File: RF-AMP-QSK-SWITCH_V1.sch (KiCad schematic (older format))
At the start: 41 parts, among them J1 TRX, J2 AMP_IN, J3 ANT, J4 AMP_OUT

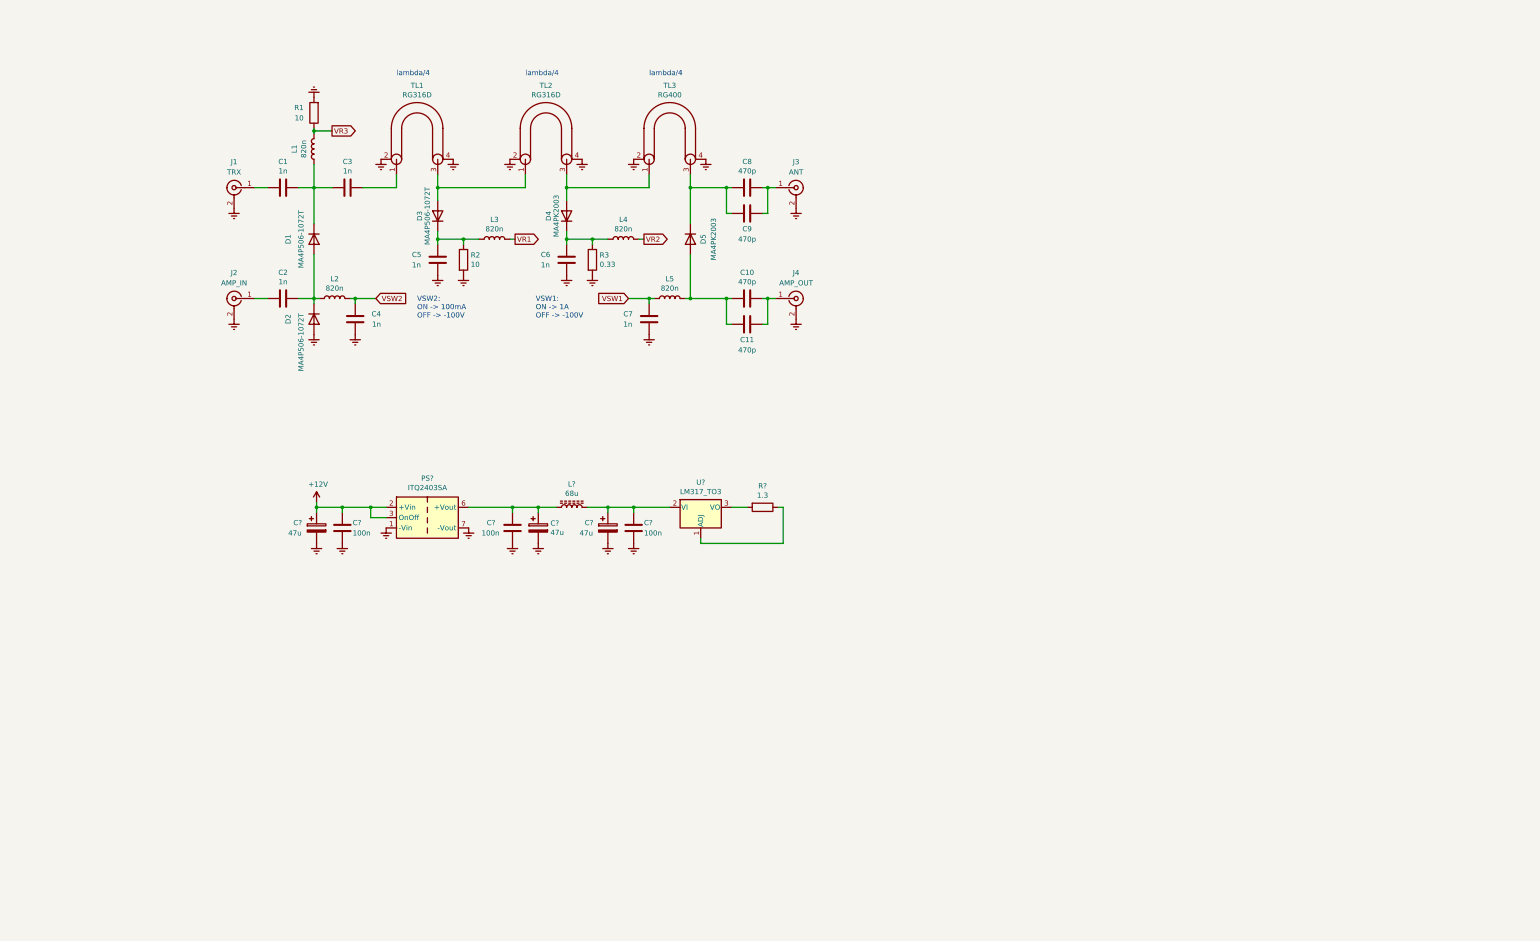
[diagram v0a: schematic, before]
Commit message: initial commit
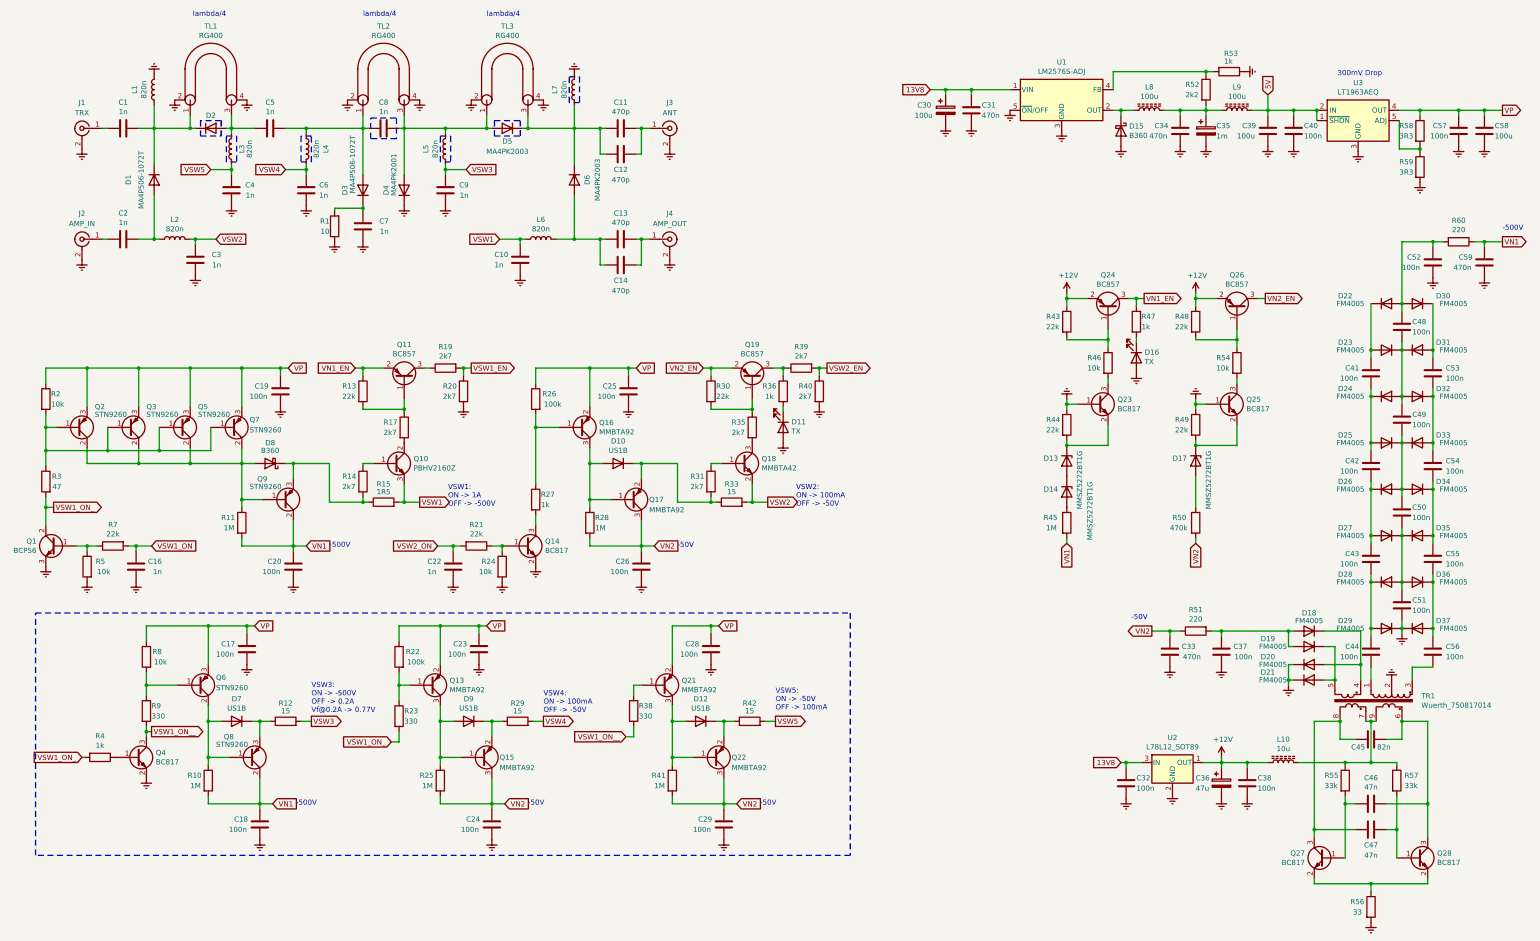
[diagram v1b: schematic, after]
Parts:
- removed C?: 47u, symbol Device:CP
- removed C?: 100n, symbol Device:C
- removed L?: 68u, symbol Device:L_Core_Ferrite
- removed PS?: ITQ2403SA, Converter_DCDC:Converter_DCDC_XP_POWER-ITxxxxxS_THT, symbol Converter_DCDC:ITQ2403SA
- removed R?: 1.3, symbol Device:R
- removed U?: LM317_TO3, Package_TO_SOT_THT:TO-3, symbol Regulator_Linear:LM317_TO3
- added C16, C22: 1n, Capacitor_SMD:C_0805_2012Metric, symbol Device:C
- added C17, C19, C23, C24, C25, C26, C28, C29, C32, C38, C40, C57: 100n, Capacitor_SMD:C_0805_2012Metric, symbol Device:C
- added C18, C20, C37, C41, C42, C43, C44, C48, C49, C50, C51, C52, C53, C54, C55, C56: 100n, Capacitor_SMD:C_1206_3216Metric, symbol Device:C
- added C33, C59: 470n, Capacitor_SMD:C_1206_3216Metric, symbol Device:C
- added C36: 47u, Capacitor_SMD:CP_Elec_10x10, symbol Device:CP
- added C39, C58: 100u, Capacitor_SMD:C_1210_3225Metric, symbol Device:C
- added C4, C7, C9: 1n, Capacitor_SMD:C_1210_3225Metric, symbol Device:C
- added C45: 82n, Capacitor_SMD:C_0805_2012Metric, symbol Device:C
- added C46, C47: 47n, Capacitor_SMD:C_0805_2012Metric, symbol Device:C
- added D10, D12, D7, D9: US1B, Diode_SMD:D_SMA, symbol Diode:US1B
- added D11, D16: TX, LED_THT:LED_D3.0mm, symbol Device:LED
- added D13, D14, D17: MMSZ5272BT1G, Diode_SMD:D_SOD-123, symbol Diode:BZD27Cxx
- added D15, D8: B360, Diode_SMD:D_SMC, symbol Diode:B360
- added D18, D19, D20, D21, D22, D23, D24, D25, D26, D27, D28, D29, D30, D31, D32, D33, D34, D35, D36, D37: FM4005, Diode_SMD:D_SMA, symbol Diode:MRA4006T3G
- added D5: MA4PK2003, RF-AMP-QSK-SWITCH_V1:MA4PK200x, symbol Device:D
- added L10: 10u, Inductor_SMD:L_1210_3225Metric, symbol Device:L_Core_Ferrite
- added L5, L7: 820n, RF-AMP-QSK-SWITCH_V1:Air_Coil_1, symbol Device:L
- added L8, L9: 100u, Inductor_SMD:L_Bourns_SRR1210A, symbol Device:L_Core_Ferrite
- added Q1: BCP56, Package_TO_SOT_SMD:SOT-223-3_TabPin2, symbol Transistor_BJT:BCP56
- added Q10: PBHV2160Z, Package_TO_SOT_SMD:SOT-223-3_TabPin2, symbol Transistor_BJT:PZTA42
- added Q11, Q19, Q24, Q26: BC857, Package_TO_SOT_SMD:SOT-23, symbol Transistor_BJT:BC857
- added Q13, Q15, Q16, Q17, Q21, Q22: MMBTA92, Package_TO_SOT_SMD:SOT-23, symbol Transistor_BJT:MMBTA92
- added Q14, Q23, Q25, Q27, Q28, Q4: BC817, Package_TO_SOT_SMD:SOT-23, symbol Transistor_BJT:BC817
- added Q18: MMBTA42, Package_TO_SOT_SMD:SOT-23, symbol Transistor_BJT:MMBTA42
- added Q2, Q3, Q5, Q6, Q7, Q8, Q9: STN9260, Package_TO_SOT_SMD:SOT-223-3_TabPin2, symbol Transistor_BJT:BD912
- added R10, R11, R25, R28, R41, R45: 1M, Resistor_SMD:R_0805_2012Metric, symbol Device:R
- added R12, R29, R33, R42: 15, Resistor_SMD:R_2512_6332Metric, symbol Device:R
- added R13, R21, R30, R43, R44, R48, R49, R7: 22k, Resistor_SMD:R_0805_2012Metric, symbol Device:R
- added R14, R17, R19, R20, R31, R35, R39, R40: 2k7, Resistor_SMD:R_0805_2012Metric, symbol Device:R
- added R15: 1R5, Resistor_SMD:R_Shunt_Vishay_WSR2_WSR3, symbol Device:R
- added R22, R26: 100k, Resistor_SMD:R_0805_2012Metric, symbol Device:R
- added R23, R38, R9: 330, Resistor_SMD:R_0805_2012Metric, symbol Device:R
- added R24, R46, R5, R54, R8: 10k, Resistor_SMD:R_0805_2012Metric, symbol Device:R
- added R27, R36, R4, R47, R53: 1k, Resistor_SMD:R_0805_2012Metric, symbol Device:R
- added R50: 470k, Resistor_SMD:R_0805_2012Metric, symbol Device:R
- added R51, R60: 220, Resistor_SMD:R_0805_2012Metric, symbol Device:R
- added R52: 2k2, Resistor_SMD:R_0805_2012Metric, symbol Device:R
- added R55, R57: 33k, Resistor_SMD:R_0805_2012Metric, symbol Device:R
- added R56: 33, Resistor_SMD:R_0805_2012Metric, symbol Device:R
- added R58, R59: 3R3, Resistor_SMD:R_0805_2012Metric, symbol Device:R
- added TR1: Wuerth_750817014, RF-AMP-QSK-SWITCH_V1:Transformer_Wuerth_750817014, symbol RF-AMP:Wuerth_750817014
- added U1: LM2576S-ADJ, Package_TO_SOT_SMD:TO-263-5_TabPin3, symbol Regulator_Switching:LM2576S-ADJ
- added U2: L78L12_SOT89, Package_TO_SOT_SMD:SOT-89-3, symbol Regulator_Linear:L78L12_SOT89
- added U3: LT1963AEQ, Package_TO_SOT_SMD:TO-263-5_TabPin3, symbol Regulator_Linear:LT1963AEQ
- C1, C2, C5, C6: footprint (none) -> Capacitor_SMD:C_1210_3225Metric
- C10: renamed from C7; footprint (none) -> Capacitor_SMD:C_1210_3225Metric
- C11: renamed from C8; footprint (none) -> Capacitor_SMD:C_1210_3225Metric
- C12: renamed from C9; footprint (none) -> Capacitor_SMD:C_1210_3225Metric
- C13: renamed from C10; footprint (none) -> Capacitor_SMD:C_1210_3225Metric
- C14: renamed from C11; footprint (none) -> Capacitor_SMD:C_1210_3225Metric
- C3: renamed from C4; footprint (none) -> Capacitor_SMD:C_1210_3225Metric
- C30: renamed from C?; value 47u -> 100u; footprint (none) -> Capacitor_SMD:CP_Elec_10x10
- C31, C34: renamed from C?; value 100n -> 470n; footprint (none) -> Capacitor_SMD:C_0805_2012Metric
- C35: renamed from C?; value 47u -> 1m; footprint (none) -> Capacitor_SMD:CP_Elec_10x10
- C8: renamed from C3; footprint (none) -> Capacitor_SMD:C_1210_3225Metric
- D1, D2, D3: footprint (none) -> Diode_SMD:D_1210_3225Metric
- D4: value MA4PK2003 -> MA4PK2001; footprint (none) -> RF-AMP-QSK-SWITCH_V1:MA4PK200x
- D6: renamed from D5; footprint (none) -> RF-AMP-QSK-SWITCH_V1:MA4PK200x
- J1, J2, J3, J4: footprint (none) -> RF-AMP-QSK-SWITCH_V1:N_connector_panel_small_flange
- L1, L2, L3, L4: footprint (none) -> RF-AMP-QSK-SWITCH_V1:Air_Coil_1
- L6: renamed from L5; footprint (none) -> RF-AMP-QSK-SWITCH_V1:Air_Coil_1
- R1: footprint (none) -> Resistor_SMD:R_1210_3225Metric
- R2: value 10 -> 10k; footprint (none) -> Resistor_SMD:R_0805_2012Metric
- R3: value 0.33 -> 47; footprint (none) -> Resistor_SMD:R_1206_3216Metric
- TL1, TL2: value RG316D -> RG400
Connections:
- net VR2 is gone; now on an unnamed net: L4.2
- net VR3 is gone; now on net Earth: L1.2, R1.1
- net +12V: now also C36.1, C38.2, L10.1, Q24.2 (E), Q26.2 (E), R43.1, R48.1, U2.1 (OUT); no longer C30.1, C31.2
- net Earth: now also D4.1 (K), C16.1, C17.1, C18.1, C19.1, C20.1, C22.1, C23.1, C24.1, C25.1, C26.1, C28.1, C29.1, C32.1, C33.1, C36.2, C37.1, C38.1, C39.1, C4.1, C40.1, C51.1, C52.1, C57.1, C58.1, C59.1, C7.1, C9.1, D11.2 (A), D15.2 (A), D16.2 (A), D20.1 (K), D21.1 (K), D29.1 (K), D37.1 (K), L7.2, Q1.3 (E), Q14.2 (E), Q23.1 (B), Q25.1 (B), Q4.2 (E), R20.2, R24.2, R40.2, R44.1, R49.1, R5.2, R53.1, R56.2, R59.2, TR1.2, U1.3 (GND), U1.5 (~ON~/OFF), U2.2 (GND), U3.3 (GND); no longer C5.1, D2.2 (A), R1.2, R2.2, R3.2
- net VSW1: now also Q10.3 (E), R15.2
- net VSW2: now also Q18.2 (E), R33.2
- net at C11.1, C12.1, D6.1 (K)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: now also D5.1 (K), L7.1
- net at C1.1, D1.1 (K), L1.1: now also D2.1 (K), TL1.1 (IC1); no longer C8.2
- net at C8.1: now also D4.2 (A), TL2.3 (IC1), TL3.1 (IC1), D5.2 (A), L5.2; no longer TL1.1 (IC1)
- net at D3.2 (A), TL2.1 (IC1): now also C5.1, C8.2; no longer TL1.3 (IC1)
- net VSW4: now reaches C6.2, L4.1
- net VSW4: now also R29.2; no longer D4.1 (K), R3.1
- net at C2.1, D1.2 (A), L2.2: no longer D2.1 (K)
- net at C34.2, C35.1: now also L8.2, L9.1, R52.2
- net VR1: no longer names the net of L3.2
- net VR1: now also C5.2, D2.2 (A), TL1.3 (IC1)
- new net: C7.2, D3.1 (K), R1.2
- new net: D15.1 (K), L8.1, U1.2 (OUT)
- new net: C55.1, C56.2, D36.1 (K), D37.2 (A)
- new net: R58.2, R59.1, U3.5 (ADJ)
- new net: Q27.2 (E), Q28.2 (E), R56.1
- new net: C44.1, TR1.1
- new net: C56.1, TR1.3
- new net: D18.1 (K), D20.2 (A), TR1.4
- new net: D19.1 (K), D21.2 (A), TR1.5
- new net: C45.1, C46.1, Q28.3 (C), TR1.6
- new net: L10.2, R55.1, R57.1, TR1.7, TR1.9
- new net: C45.2, C47.2, Q27.3 (C), TR1.8
- new net: Q2.1 (B), Q3.1 (B), Q5.1 (B), Q7.1 (B), R2.2, R3.1
- new net: D8.2 (A), Q2.2 (C), Q3.2 (C), Q5.2 (C), Q7.2 (C), Q9.1 (B), R11.1
- new net: D8.1 (K), Q9.3 (E), R14.2, R15.1
- new net: Q1.1 (B), R5.1, R7.1
- new net: R52.1, R53.2, U1.4 (FB)
- new net: C47.1, Q28.1 (B), R57.2
- new net: C37.2, D18.2 (A), D19.2 (A), R51.2
- new net: C46.2, Q27.1 (B), R55.2
- new net: C48.2, C52.2, D22.2 (A), D30.2 (A), R60.2
- new net: Q19.3 (C), R36.1, R39.1
- new net: D11.1 (K), R36.2
- new net: D13.1 (K), Q23.2 (E), R44.2
- new net: D13.2 (A), D14.1 (K)
- new net: Q11.1 (B), R13.2, R17.1
- new net: Q24.1 (B), R43.2, R46.1
- new net: Q23.3 (C), R46.2
- new net: D16.1 (K), R47.2
- new net: Q10.1 (B), R14.1
- new net: Q10.2 (C), R17.2
- new net: D14.2 (A), R45.1
- new net: D10.2 (A), Q16.3 (C), Q17.1 (B), R28.1
- new net: Q14.1 (B), R21.1, R24.1
- new net: Q16.1 (B), R26.2, R27.1
- new net: Q14.3 (C), R27.2
- new net: Q11.3 (C), R19.1
- new net: C43.1, C44.2, D28.1 (K), D29.2 (A)
- new net: D10.1 (K), Q17.2 (E), R31.2, R33.1
- new net: Q18.1 (B), R31.1
- new net: Q19.1 (B), R30.2, R35.1
- new net: Q18.3 (C), R35.2
- new net: D17.1 (K), Q25.2 (E), R49.2
- new net: D17.2 (A), R50.1
- new net: Q26.1 (B), R48.2, R54.1
- new net: Q25.3 (C), R54.2
- new net: C50.1, C51.2, D27.1 (K), D28.2 (A), D35.1 (K), D36.2 (A)
- new net: D7.2 (A), Q6.2 (C), Q8.1 (B), R10.1
- new net: Q4.1 (B), R4.1
- new net: D7.1 (K), Q8.3 (E), R12.1
- new net: Q6.1 (B), R8.2, R9.1
- new net: C54.1, C55.2, D34.1 (K), D35.2 (A)
- new net: C42.1, C43.2, D26.1 (K), D27.2 (A)
- new net: C49.1, C50.2, D25.1 (K), D26.2 (A), D33.1 (K), D34.2 (A)
- new net: C53.1, C54.2, D32.1 (K), D33.2 (A)
- new net: C41.1, C42.2, D24.1 (K), D25.2 (A)
- new net: C48.1, C49.2, D23.1 (K), D24.2 (A), D31.1 (K), D32.2 (A)
- new net: C53.2, D30.1 (K), D31.2 (A)
- new net: C41.2, D22.1 (K), D23.2 (A)
- new net: D9.2 (A), Q13.3 (C), Q15.1 (B), R25.1
- new net: Q13.1 (B), R22.2, R23.1
- new net: D9.1 (K), Q15.2 (E), R29.1
- new net: D12.2 (A), Q21.3 (C), Q22.1 (B), R41.1
- new net: Q21.1 (B), R38.1
- new net: D12.1 (K), Q22.2 (E), R42.1
- new net 13V8: C30.1, C31.2, C32.2, U1.1 (VIN), U2.3 (IN)
- new net 5V: C39.2, C40.2, L9.2, U3.1 (~SHDN), U3.2 (IN)
- new net VN1: C18.2, C20.2, C59.2, Q8.2 (C), Q9.2 (C), R10.2, R11.2, R45.2, R60.1
- new net VN1_EN: Q11.2 (E), Q24.3 (C), R13.1, R47.1
- new net VN2: C24.2, C26.2, C29.2, C33.2, Q15.3 (C), Q17.3 (C), Q22.3 (C), R25.2, R28.2, R41.2, R50.2, R51.1
- new net VN2_EN: Q19.2 (E), Q26.3 (C), R30.1
- new net VP: C17.2, C19.2, C23.2, C25.2, C28.2, C57.2, C58.2, Q13.2 (E), Q16.2 (E), Q2.3 (E), Q21.2 (E), Q3.3 (E), Q5.3 (E), Q6.3 (E), Q7.3 (E), R2.1, R22.1, R26.1, R58.1, R8.1, U3.4 (OUT)
- new net VSW1_EN: R19.2, R20.1
- new net VSW1_ON: C16.2, R7.2
- new net VSW1_ON_: Q1.2 (C), Q1.4 (C), R23.2, R3.2, R4.2
- new net VSW1_ON__: Q4.3 (C), R38.2, R9.2
- new net VSW2_EN: R39.2, R40.1
- new net VSW2_ON: C22.2, R21.2
- new net VSW3: C9.2, L5.1, R12.2
- new net VSW5: C4.2, L3.1, R42.2
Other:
- note added: "-500V"
- note added: "-50V"
- note added: "300mV Drop"
- note added: "VSW1:\nON -> 1A\nOFF -> -500V"
- note added: "VSW2:\nON -> 100mA\nOFF -> -50V"
- note added: "VSW3:\nON -> -500V\nOFF -> 0.2A\nVf@0.2A -> 0.77V"
- note added: "VSW4:\nON -> 100mA\nOFF -> -50V"
- note added: "VSW5:\nON -> -50V\nOFF -> 100mA"
- note removed: "VSW1:\nON -> 1A\nOFF -> -100V"
- note removed: "VSW2:\nON -> 100mA\nOFF -> -100V"
- moved on the sheet: C1, C10, C11, C12, C13, C14, C2, C3, C30, C31, C34, C35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
